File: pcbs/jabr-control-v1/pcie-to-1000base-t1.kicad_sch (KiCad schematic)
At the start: 0 parts

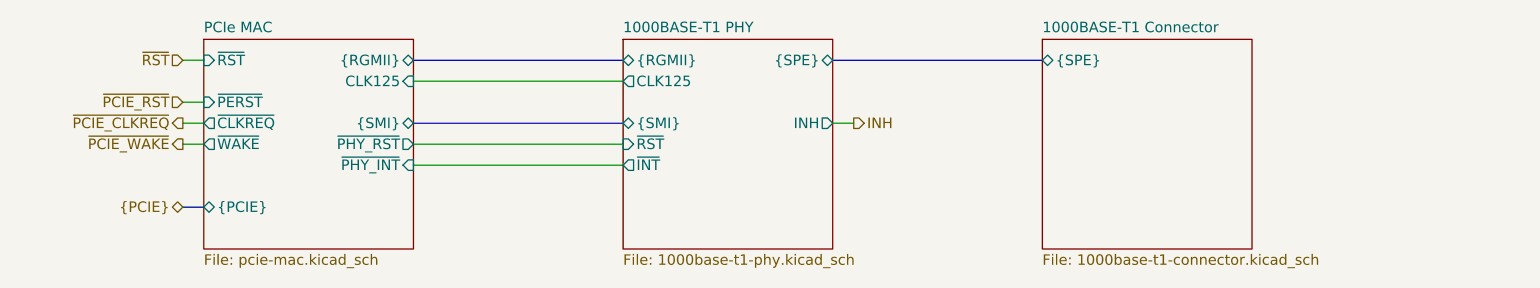
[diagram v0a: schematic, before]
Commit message: Various small updates
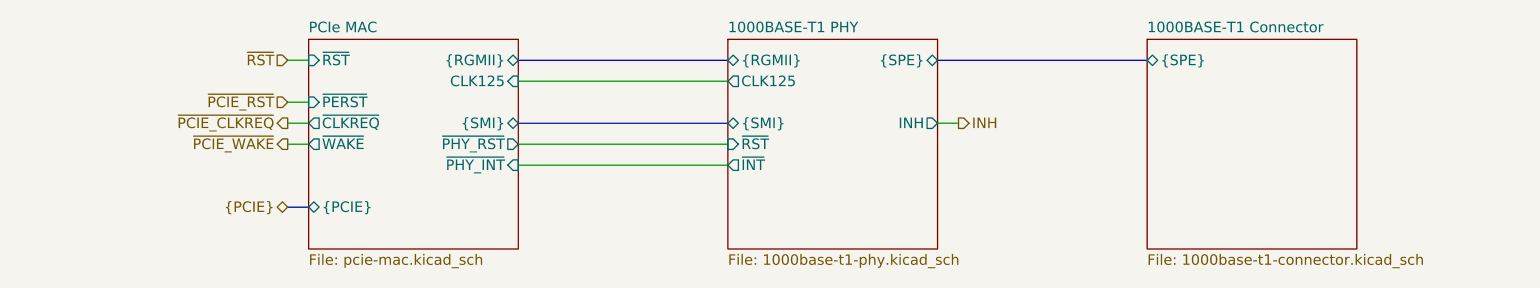
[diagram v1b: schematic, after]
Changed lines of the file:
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@@
 	(bus
 		(pts
-			(xy 73.66 96.52) (xy 76.2 96.52)
-		)
-		(stroke
-			(width 0)
-			(type default)
-		)
-	)
-	(wire
-		(pts
-			(xy 73.66 88.9) (xy 76.2 88.9)
-		)
-		(stroke
-			(width 0)
-			(type default)
-		)
-	)
-	(wire
-		(pts
-			(xy 73.66 83.82) (xy 76.2 83.82)
-		)
-		(stroke
-			(width 0)
-			(type default)
-		)
-	)
-	(wire
-		(pts
-			(xy 73.66 86.36) (xy 76.2 86.36)
-		)
-		(stroke
-			(width 0)
-			(type default)
-		)
-	)
-	(wire
-		(pts
-			(xy 152.4 86.36) (xy 154.94 86.36)
+			(xy 86.36 96.52) (xy 88.9 96.52)
+		)
+		(stroke
+			(width 0)
+			(type default)
+		)
+	)
+	(wire
+		(pts
+			(xy 86.36 88.9) (xy 88.9 88.9)
+		)
+		(stroke
+			(width 0)
+			(type default)
+		)
+	)
+	(wire
+		(pts
+			(xy 86.36 83.82) (xy 88.9 83.82)
+		)
+		(stroke
+			(width 0)
+			(type default)
+		)
+	)
+	(wire
+		(pts
+			(xy 86.36 86.36) (xy 88.9 86.36)
+		)
+		(stroke
+			(width 0)
+			(type default)
+		)
+	)
+	(wire
+		(pts
+			(xy 165.1 86.36) (xy 167.64 86.36)
 		)
 		(stroke
@@
 	(bus
 		(pts
-			(xy 101.6 86.36) (xy 127 86.36)
-		)
-		(stroke
-			(width 0)
-			(type default)
-		)
-	)
-	(wire
-		(pts
-			(xy 101.6 88.9) (xy 127 88.9)
+			(xy 114.3 86.36) (xy 139.7 86.36)
+		)
+		(stroke
+			(width 0)
+			(type default)
+		)
+	)
+	(wire
+		(pts
+			(xy 114.3 88.9) (xy 139.7 88.9)
 		)
 		(stroke
@@
 	(bus
 		(pts
-			(xy 101.6 78.74) (xy 127 78.74)
-		)
-		(stroke
-			(width 0)
-			(type default)
-		)
-	)
-	(wire
-		(pts
-			(xy 73.66 78.74) (xy 76.2 78.74)
-		)
-		(stroke
-			(width 0)
-			(type default)
-		)
-	)
-	(wire
-		(pts
-			(xy 101.6 91.44) (xy 127 91.44)
+			(xy 114.3 78.74) (xy 139.7 78.74)
+		)
+		(stroke
+			(width 0)
+			(type default)
+		)
+	)
+	(wire
+		(pts
+			(xy 86.36 78.74) (xy 88.9 78.74)
+		)
+		(stroke
+			(width 0)
+			(type default)
+		)
+	)
+	(wire
+		(pts
+			(xy 114.3 91.44) (xy 139.7 91.44)
 		)
 		(stroke
@@
 	(bus
 		(pts
-			(xy 152.4 78.74) (xy 177.8 78.74)
-		)
-		(stroke
-			(width 0)
-			(type default)
-		)
-	)
-	(wire
-		(pts
-			(xy 101.6 81.28) (xy 127 81.28)
+			(xy 165.1 78.74) (xy 190.5 78.74)
+		)
+		(stroke
+			(width 0)
+			(type default)
+		)
+	)
+	(wire
+		(pts
+			(xy 114.3 81.28) (xy 139.7 81.28)
 		)
 		(stroke
@@
 	(hierarchical_label "~{PCIE_WAKE}"
 		(shape output)
-		(at 73.66 88.9 180)
+		(at 86.36 88.9 180)
 		(effects
 			(font
@@
 	(hierarchical_label "~{PCIE_CLKREQ}"
 		(shape output)
-		(at 73.66 86.36 180)
+		(at 86.36 86.36 180)
 		(effects
 			(font
@@
 	(hierarchical_label "~{RST}"
 		(shape input)
-		(at 73.66 78.74 180)
+		(at 86.36 78.74 180)
 		(effects
 			(font
@@
 	(hierarchical_label "INH"
 		(shape output)
-		(at 154.94 86.36 0)
+		(at 167.64 86.36 0)
 		(effects
 			(font
@@
 	(hierarchical_label "~{PCIE_RST}"
 		(shape input)
-		(at 73.66 83.82 180)
+		(at 86.36 83.82 180)
 		(effects
 			(font
@@
 	(hierarchical_label "{PCIE}"
 		(shape bidirectional)
-		(at 73.66 96.52 180)
+		(at 86.36 96.52 180)
 		(effects
 			(font
@@
 	)
 	(sheet
-		(at 76.2 76.2)
+		(at 88.9 76.2)
 		(size 25.4 25.4)
 		(exclude_from_sim no)
@@
 		)
 		(property "Sheetname" "PCIe MAC"
-			(at 76.2 75.4884 0)
+			(at 88.9 75.4884 0)
 			(effects
 				(font
@@
 		)
 		(property "Sheetfile" "pcie-mac.kicad_sch"
-			(at 76.2 102.1846 0)
+			(at 88.9 102.1846 0)
 			(effects
 				(font
@@
 		)
 		(pin "{PCIE}" bidirectional
-			(at 76.2 96.52 180)
+			(at 88.9 96.52 180)
 			(effects
 				(font
@@
 		)
 		(pin "~{RST}" input
-			(at 76.2 78.74 180)
+			(at 88.9 78.74 180)
 			(effects
 				(font
@@
 		)
 		(pin "~{CLKREQ}" output
-			(at 76.2 86.36 180)
+			(at 88.9 86.36 180)
 			(effects
 				(font
@@
 		)
 		(pin "~{WAKE}" output
-			(at 76.2 88.9 180)
+			(at 88.9 88.9 180)
 			(effects
 				(font
@@
 		)
 		(pin "{RGMII}" bidirectional
-			(at 101.6 78.74 0)
+			(at 114.3 78.74 0)
 			(effects
 				(font
@@
 		)
 		(pin "{SMI}" bidirectional
-			(at 101.6 86.36 0)
+			(at 114.3 86.36 0)
 			(effects
 				(font
@@
 		)
 		(pin "~{PHY_INT}" input
-			(at 101.6 91.44 0)
+			(at 114.3 91.44 0)
 			(effects
 				(font
@@
 		)
 		(pin "~{PHY_RST}" output
-			(at 101.6 88.9 0)
+			(at 114.3 88.9 0)
 			(effects
 				(font
@@
 		)
 		(pin "CLK125" input
-			(at 101.6 81.28 0)
+			(at 114.3 81.28 0)
 			(effects
 				(font
@@
 		)
 		(pin "~{PERST}" input
-			(at 76.2 83.82 180)
+			(at 88.9 83.82 180)
 			(effects
 				(font
@@
 	)
 	(sheet
-		(at 177.8 76.2)
+		(at 190.5 76.2)
 		(size 25.4 25.4)
 		(exclude_from_sim no)
@@
 		)
 		(property "Sheetname" "1000BASE-T1 Connector"
-			(at 177.8 75.4884 0)
+			(at 190.5 75.4884 0)
 			(effects
 				(font
@@
 		)
 		(property "Sheetfile" "1000base-t1-connector.kicad_sch"
-			(at 177.8 102.1846 0)
+			(at 190.5 102.1846 0)
 			(effects
 				(font
@@
 		)
 		(pin "{SPE}" bidirectional
-			(at 177.8 78.74 180)
+			(at 190.5 78.74 180)
 			(effects
 				(font
@@
 	)
 	(sheet
-		(at 127 76.2)
+		(at 139.7 76.2)
 		(size 25.4 25.4)
 		(exclude_from_sim no)
@@
 		)
 		(property "Sheetname" "1000BASE-T1 PHY"
-			(at 127 75.4884 0)
+			(at 139.7 75.4884 0)
 			(effects
 				(font
@@
 		)
 		(property "Sheetfile" "1000base-t1-phy.kicad_sch"
-			(at 127 102.1846 0)
+			(at 139.7 102.1846 0)
 			(effects
 				(font
@@
 		)
 		(pin "{RGMII}" bidirectional
-			(at 127 78.74 180)
+			(at 139.7 78.74 180)
 			(effects
 				(font
@@
 		)
 		(pin "{SMI}" bidirectional
-			(at 127 86.36 180)
+			(at 139.7 86.36 180)
 			(effects
 				(font
@@
 		)
 		(pin "~{INT}" output
-			(at 127 91.44 180)
+			(at 139.7 91.44 180)
 			(effects
 				(font
@@
 		)
 		(pin "~{RST}" input
-			(at 127 88.9 180)
+			(at 139.7 88.9 180)
 			(effects
 				(font
@@
 		)
 		(pin "CLK125" output
-			(at 127 81.28 180)
+			(at 139.7 81.28 180)
 			(effects
 				(font
@@
 		)
 		(pin "{SPE}" bidirectional
-			(at 152.4 78.74 0)
+			(at 165.1 78.74 0)
 			(effects
 				(font
@@
 		)
 		(pin "INH" output
-			(at 152.4 86.36 0)
-			(effects
-				(font
+			(at 165.1 86.36 0)
+			(effects
+				(font
